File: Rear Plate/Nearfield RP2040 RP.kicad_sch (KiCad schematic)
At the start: 8 parts

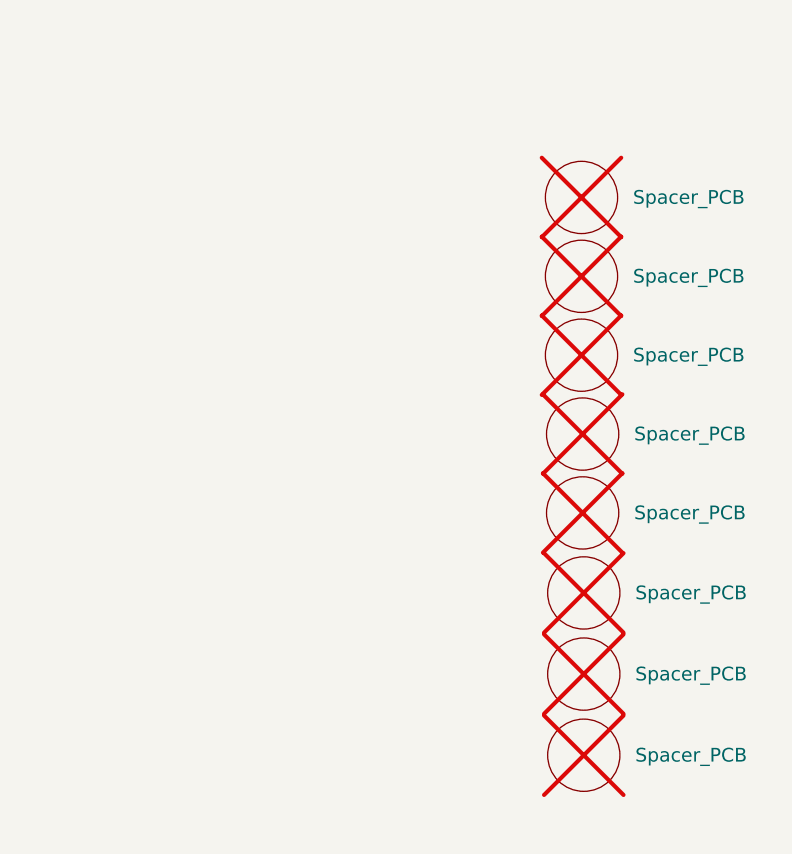
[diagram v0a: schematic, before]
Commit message: V1.00
Full design ready
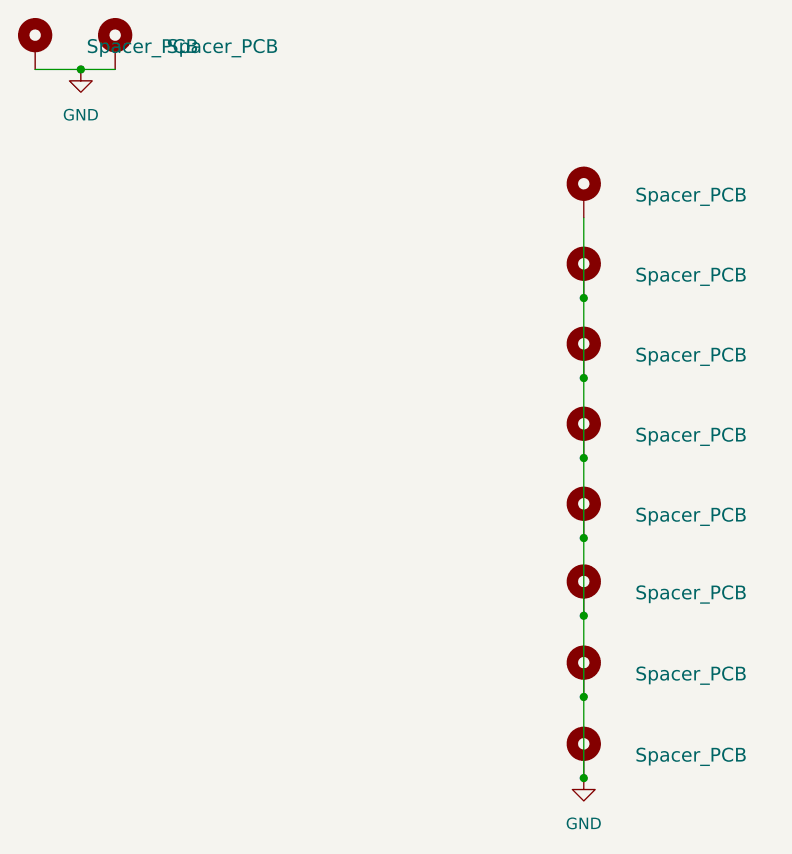
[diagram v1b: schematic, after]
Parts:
- added H10 (x2): Spacer_PCB, Keyboard_Plate:Spacer_Plate_Grounded_m3, symbol Keyboard_Plate:Spacer_Plate_Grounded
- H1, H10, H2, H3, H6, H7, H8, H9: footprint Keyboard_Plate:Spacer Plate hole -> Keyboard_Plate:Spacer_Plate_Grounded; symbol Keyboard_Plate:Spacer_PCB -> Keyboard_Plate:Spacer_Plate_Grounded; now fitted
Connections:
- new net GND: H1.1, H10.1, H10.1, H10.1, H2.1, H3.1, H6.1, H7.1, H8.1, H9.1
